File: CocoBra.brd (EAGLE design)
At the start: 41.9 x 46.9 mm, 22 parts, among them U3 ATTINY84

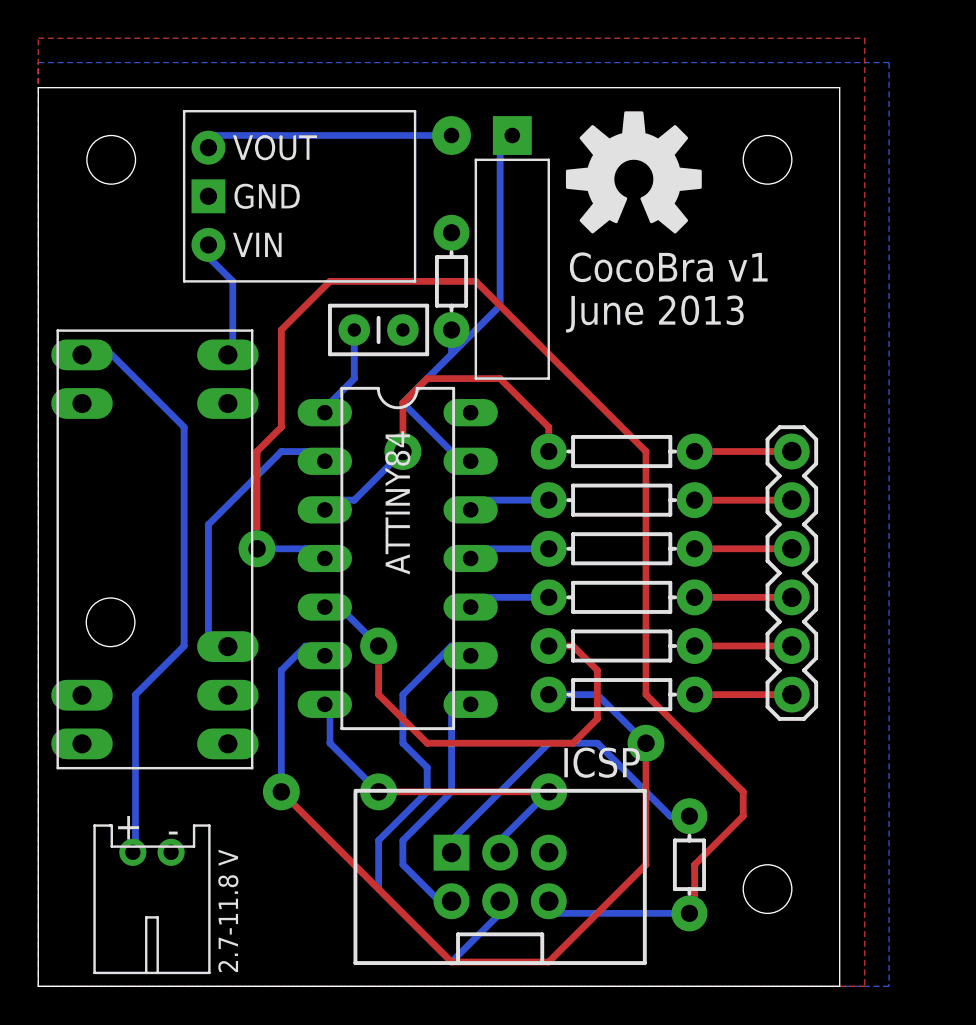
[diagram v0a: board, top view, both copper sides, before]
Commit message: tagged v1
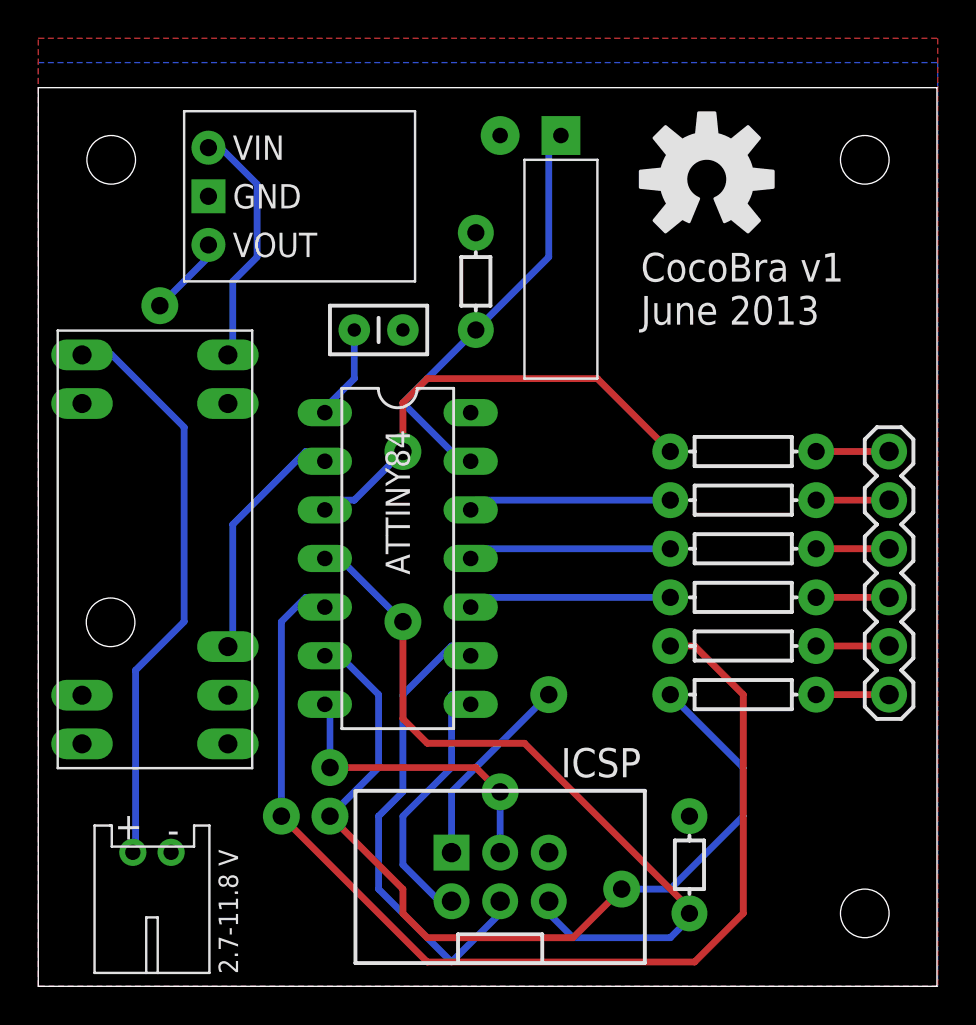
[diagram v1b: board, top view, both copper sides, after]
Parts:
- moved R2 6.35 mm to (36.8, 17.8)
- moved R3 6.35 mm to (36.8, 27.9)
- moved R4 6.35 mm to (36.8, 15.2)
- moved R5 6.35 mm to (36.8, 20.3)
- moved R6 6.35 mm to (36.8, 22.9)
- moved R7 6.35 mm to (36.8, 25.4)
- moved STANDOFF2 5.24 mm to (43.2, 3.81)
- moved JP2 5.08 mm to (44.5, 27.9)
- moved STANDOFF1 5.08 mm to (43.2, 43.2)
- moved U$1 3.81 mm to (34.9, 42.2)
- moved U$3 2.54 mm to (29.2, 43.2)
- moved R8 1.27 mm to (22.9, 36.8)
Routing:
- net RST: track 75.2 -> 40.3 mm
- net N$1: track 25.3 -> 57.7 mm
- net VCC: track 35.3 -> 19.5 mm, vias 0 -> 2
- net VOUT: track 6.50 -> 13.9 mm
- net N$6: track 4.39 -> 10.7 mm
- net N$5: track 4.39 -> 10.7 mm
- net N$4: track 4.39 -> 10.7 mm
- net N$2: track 18.4 -> 24.1 mm
- net MOSI: track 19.8 -> 17.0 mm
- net OFF: track 15.1 -> 13.1 mm
- net JP7: track 5.08 -> 3.81 mm
- net JP6: track 5.08 -> 3.81 mm
- net JP5: track 5.08 -> 3.81 mm
- net JP4: track 5.08 -> 3.81 mm
- net JP3: track 5.08 -> 3.81 mm
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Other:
- board size 41.9 x 46.9 mm -> 46.9 x 46.9 mm
